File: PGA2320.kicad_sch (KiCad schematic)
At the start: 31 parts, among them J1 XH2.54-3P, J2 XH2.54-3P, J3 2P-2.54, J4 3P-2.54, P1 SDO_TO_OTHER_PGA2311, P2 CONTROLLER, Q1 BC550, Q2 BC560, U1 PGA2320

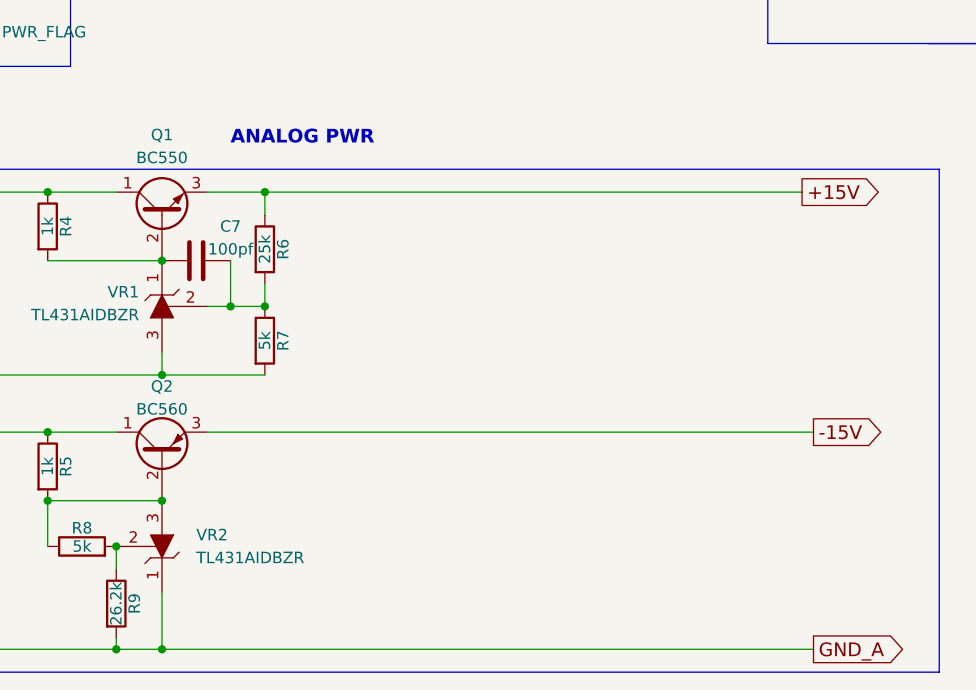
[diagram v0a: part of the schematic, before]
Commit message: add PI filter
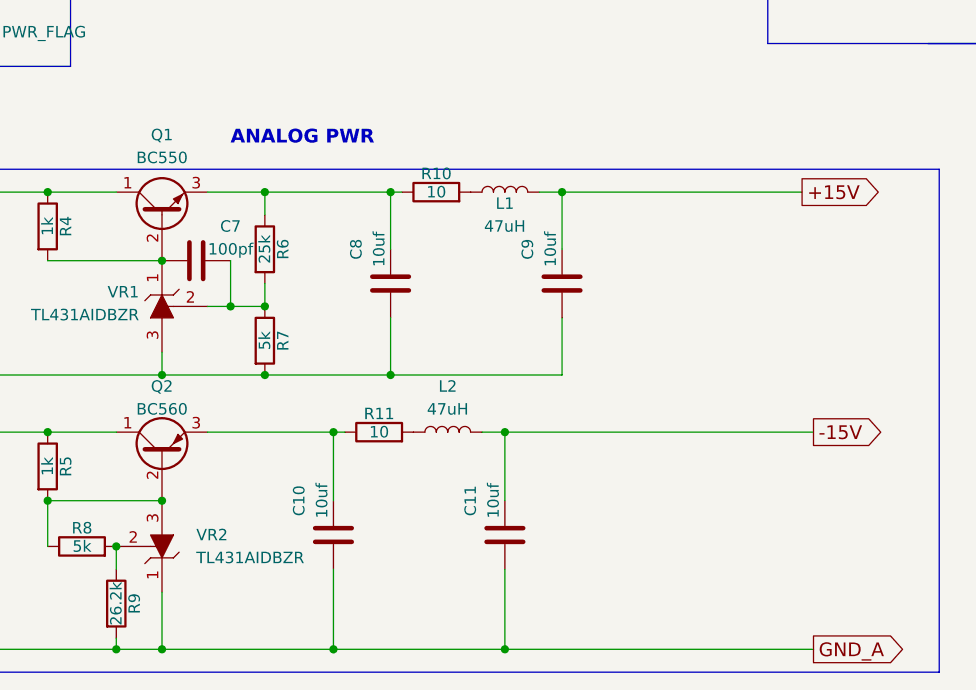
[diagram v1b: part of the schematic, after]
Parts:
- added C10, C11, C8, C9: 10uf, Capacitor_SMD:C_0805_2012Metric, symbol Device:C
- added L1, L2: 47uH, Inductor_SMD:L_0805_2012Metric, symbol Device:L
- added R10, R11: 10, Resistor_SMD:R_0805_2012Metric_Pad1.20x1.40mm_HandSolder, symbol Device:R
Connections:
- net +15V: now also C9.2, L1.2; no longer Q1.3 (E), R6.1
- net -15V: now also C11.2, L2.2; no longer Q2.3 (E)
- net GND_A: now also C10.1, C11.1, C8.1, C9.1
- new net: C10.2, Q2.3 (E), R11.1
- new net: C8.2, Q1.3 (E), R10.1, R6.1
- new net: L1.1, R10.2
- new net: L2.1, R11.2
